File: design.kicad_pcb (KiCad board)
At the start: 2 copper layers, 40 x 40 mm, 30 parts, among them J1 USB4130-GF-C, SW1 EN, SW2 IO9, U1 MCP1700-3302E_SOT23, U2 TCK108AF,LF, U3 ESP32-C3-WROOM-02-N4, U4 TTP223

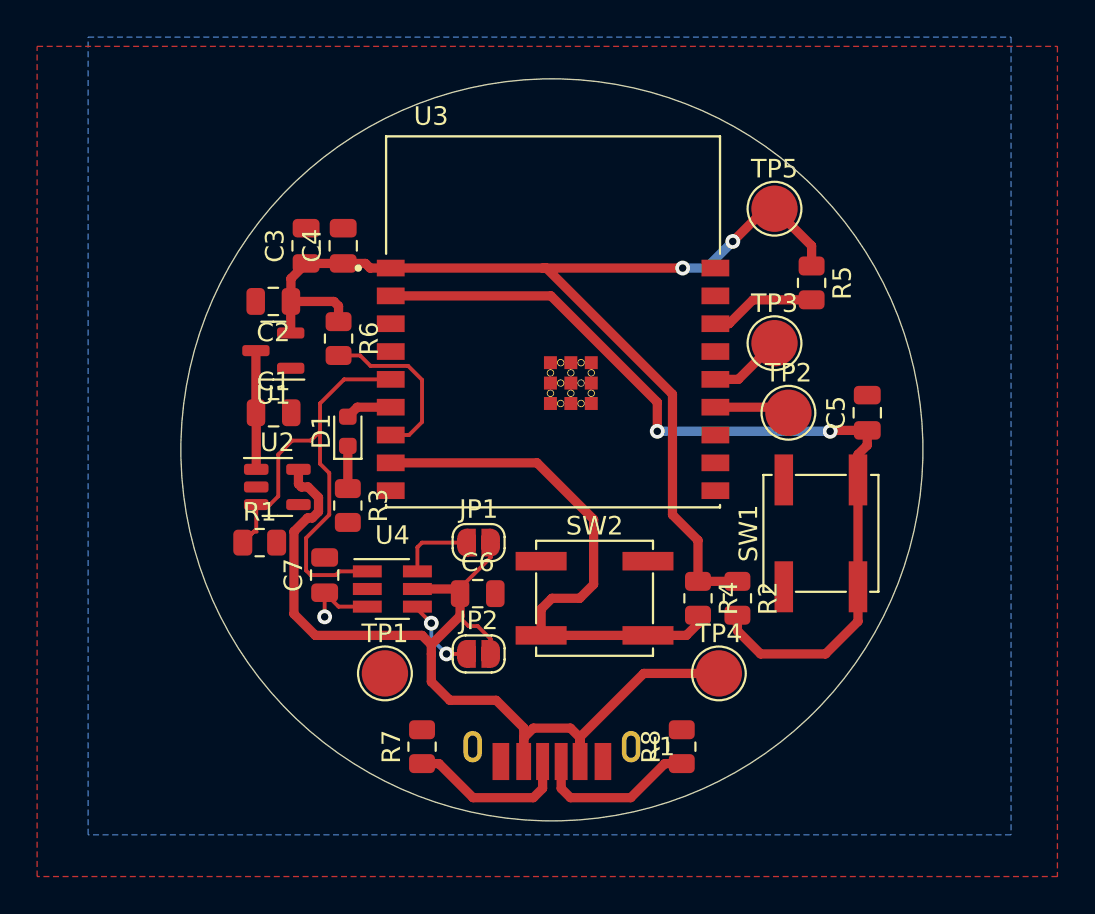
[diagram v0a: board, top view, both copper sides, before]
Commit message: PCB design
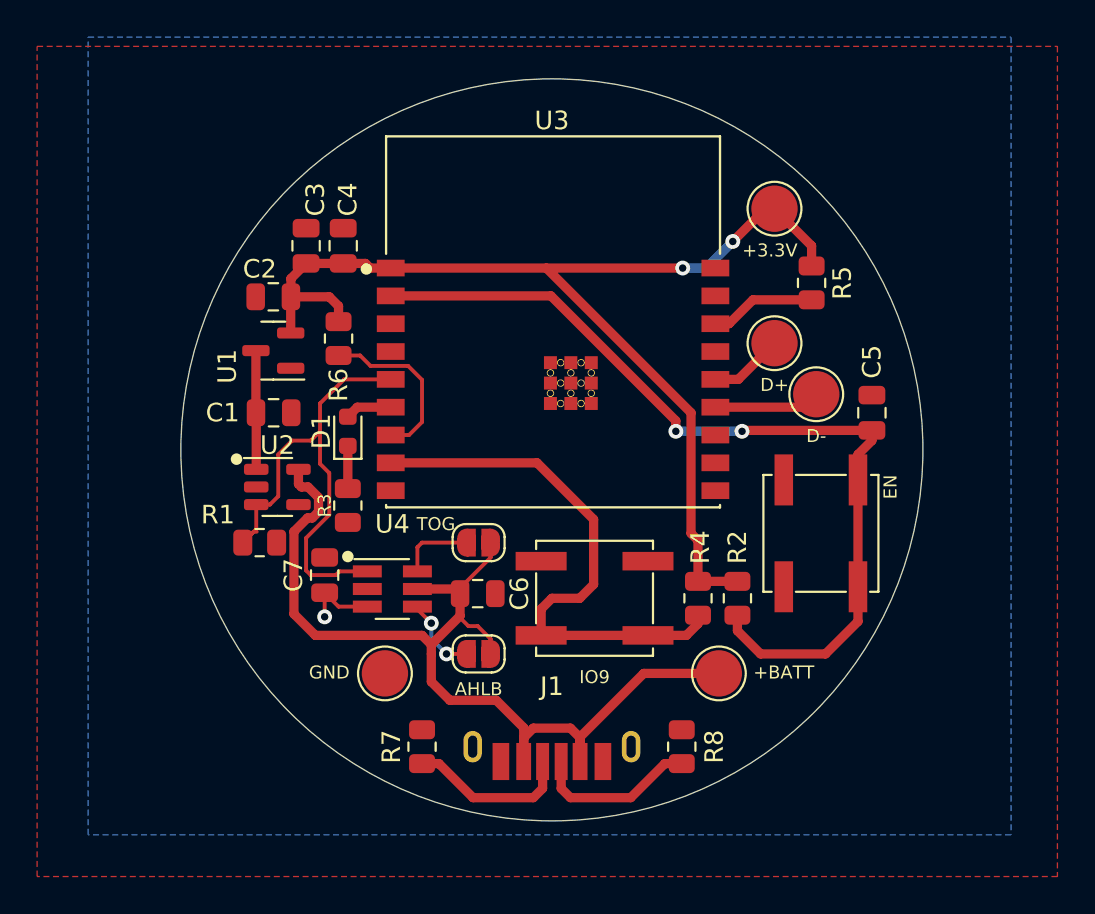
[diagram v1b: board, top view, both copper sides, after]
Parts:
- moved TP2 1.80 mm to (164.2, 97.0)
- moved C2 0.25 mm to (135.0, 91.8)
- moved C5 0.25 mm to (167.2, 98.0)
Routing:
- net D-: track 4.06 -> 5.73 mm
